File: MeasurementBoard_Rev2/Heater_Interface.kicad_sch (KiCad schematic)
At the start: 8 parts, among them CN4 Conn_01x02_Pin, CN5 Conn_01x02_Pin, CN6 Conn_01x02_Pin, CN7 Conn_01x02_Pin

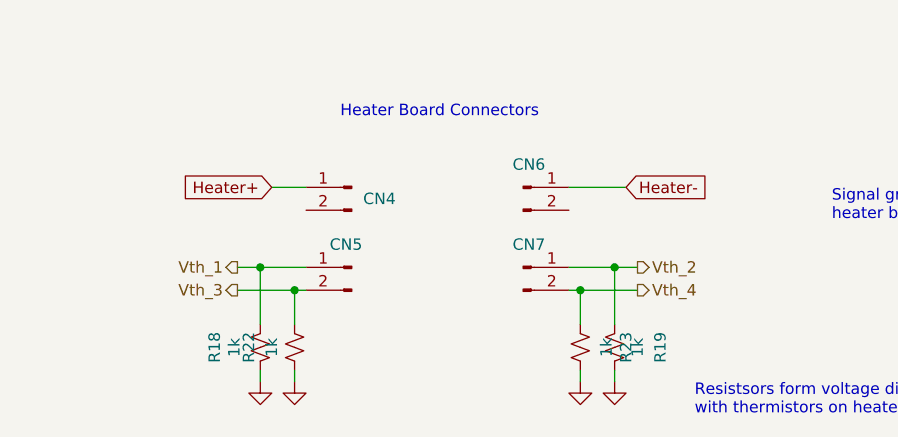
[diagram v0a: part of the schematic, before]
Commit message: Nearly Finalized Boards
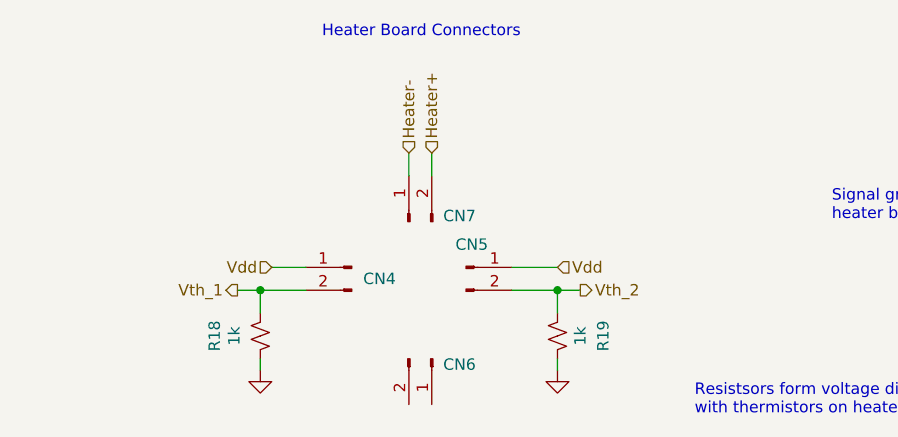
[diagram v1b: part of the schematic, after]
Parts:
- removed R22, R23: 1k, Resistor_SMD:R_0603_1608Metric_Pad0.98x0.95mm_HandSolder, symbol Device:R_Small_US
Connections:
- net Vth_3 is gone; now on net Vth_2: CN5.2 (Pin_2)
- net Vth_4 is gone; now on net Heater+: CN7.2 (Pin_2)
- net Heater+: no longer CN4.1 (Pin_1)
- net Heater-: now also CN7.1 (Pin_1); no longer CN6.1 (Pin_1)
- net Vth_1: now also CN4.2 (Pin_2); no longer CN5.1 (Pin_1)
- net Vth_2: no longer CN7.1 (Pin_1)
- new net Vdd: CN4.1 (Pin_1), CN5.1 (Pin_1)
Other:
- moved on the sheet: CN4, CN5, CN6, CN7, R18, R19
